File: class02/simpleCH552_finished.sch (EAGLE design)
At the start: 15 parts, among them U1 CH552G, X1 USBPCB

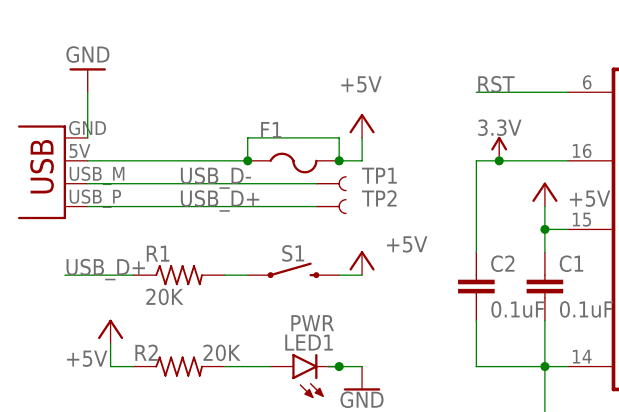
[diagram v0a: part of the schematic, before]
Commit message: remove fuse and test point
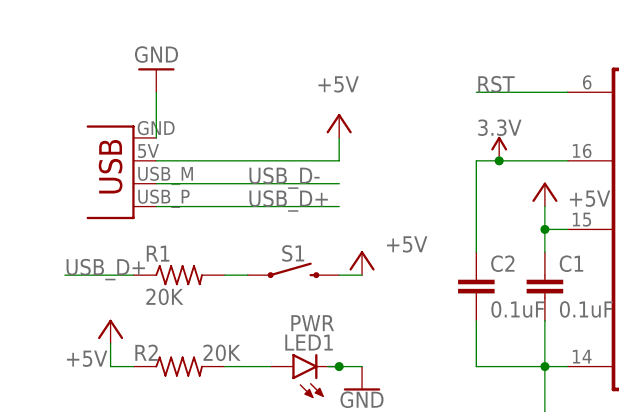
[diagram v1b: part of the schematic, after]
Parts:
- removed F1: DNP, adafruit:PTCFUSE-1206
- removed TP1, TP2: TEST-POINT3X4, SparkFun-Connectors:TEST-POINT3X4
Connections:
- net +5V: no longer F1.1, F1.2
- net USB_D+: no longer TP2.1
- net USB_D-: no longer TP1.1
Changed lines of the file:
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@@
 <attribute name="LCSC" value="C16834"/>
-</part>
-<part name="F1" library="adafruit" library_urn="urn:adsk.eagle:library:420" deviceset="PTCFUSE" device="-1206" value="DNP">
-<attribute name="LCSC" value="C151162"/>
 </part>
 <part name="GND1" library="SparkFun-PowerSymbols" library_urn="urn:adsk.eagle:library:530" deviceset="GND" device=""/>
@@
 <part name="P+4" library="supply1" library_urn="urn:adsk.eagle:library:371" deviceset="+5V" device=""/>
 <part name="P+5" library="supply1" library_urn="urn:adsk.eagle:library:371" deviceset="+5V" device=""/>
-<part name="TP1" library="SparkFun-Connectors" library_urn="urn:adsk.eagle:library:513" deviceset="TEST-POINT" device="3X4" package3d_urn="urn:adsk.eagle:package:38287/1"/>
-<part name="TP2" library="SparkFun-Connectors" library_urn="urn:adsk.eagle:library:513" deviceset="TEST-POINT" device="3X4" package3d_urn="urn:adsk.eagle:package:38287/1"/>
 <part name="S1" library="SparkFun-Switches" library_urn="urn:adsk.eagle:library:535" deviceset="MOMENTARY-SWITCH-SPST" device="-SMD-6.2MM-TALL" package3d_urn="urn:adsk.eagle:package:40172/1">
 <attribute name="LCSC" value="C557616"/>
@@
 <attribute name="VALUE" x="95.504" y="15.621" size="1.778" layer="96"/>
 </instance>
-<instance part="F1" gate="G$1" x="66.04" y="30.48" smashed="yes">
-<attribute name="LCSC" x="66.04" y="30.48" size="1.778" layer="96" display="off"/>
-<attribute name="NAME" x="62.23" y="35.56" size="1.778" layer="95"/>
-</instance>
 <instance part="GND1" gate="1" x="93.98" y="2.54" smashed="yes">
 <attribute name="VALUE" x="93.98" y="2.286" size="1.778" layer="96" align="top-center"/>
 </instance>
-<instance part="P+1" gate="1" x="73.66" y="38.1" smashed="yes">
-<attribute name="VALUE" x="71.12" y="40.64" size="1.778" layer="96"/>
+<instance part="P+1" gate="1" x="71.12" y="38.1" smashed="yes">
+<attribute name="VALUE" x="68.58" y="40.64" size="1.778" layer="96"/>
 </instance>
 <instance part="P+2" gate="1" x="93.98" y="30.48" smashed="yes">
@@
 <attribute name="LCSC" x="66.04" y="10.16" size="1.778" layer="96" rot="R90" display="off"/>
 </instance>
-<instance part="X1" gate="G$1" x="40.64" y="35.56" smashed="yes" rot="R180"/>
-<instance part="GND2" gate="1" x="43.18" y="43.18" smashed="yes" rot="R180">
-<attribute name="VALUE" x="45.72" y="45.72" size="1.778" layer="96" rot="R180"/>
+<instance part="X1" gate="G$1" x="48.26" y="35.56" smashed="yes" rot="R180"/>
+<instance part="GND2" gate="1" x="50.8" y="43.18" smashed="yes" rot="R180">
+<attribute name="VALUE" x="53.34" y="45.72" size="1.778" layer="96" rot="R180"/>
 </instance>
 <instance part="J1" gate="G$1" x="91.44" y="-20.32" smashed="yes">
@@
 <instance part="P+5" gate="1" x="73.66" y="22.86" smashed="yes">
 <attribute name="VALUE" x="76.2" y="22.86" size="1.778" layer="96"/>
-</instance>
-<instance part="TP1" gate="G$1" x="68.58" y="30.48" smashed="yes">
-<attribute name="NAME" x="73.66" y="30.48" size="1.778" layer="95" font="vector"/>
-</instance>
-<instance part="TP2" gate="G$1" x="68.58" y="27.94" smashed="yes">
-<attribute name="NAME" x="73.66" y="27.94" size="1.778" layer="95" font="vector"/>
 </instance>
 <instance part="S1" gate="G$1" x="66.04" y="20.32" smashed="yes">
@@
 <pinref part="X1" gate="G$1" pin="GND"/>
 <pinref part="GND2" gate="1" pin="GND"/>
-<wire x1="43.18" y1="35.56" x2="43.18" y2="40.64" width="0.1524" layer="91"/>
+<wire x1="50.8" y1="35.56" x2="50.8" y2="40.64" width="0.1524" layer="91"/>
 </segment>
 <segment>
@@
 <net name="USB_D-" class="0">
 <segment>
-<label x="53.34" y="30.48" size="1.778" layer="95"/>
+<label x="60.96" y="30.48" size="1.778" layer="95"/>
 <pinref part="X1" gate="G$1" pin="D-"/>
-<wire x1="68.58" y1="30.48" x2="43.18" y2="30.48" width="0.1524" layer="91"/>
-<pinref part="TP1" gate="G$1" pin="1"/>
+<wire x1="71.12" y1="30.48" x2="50.8" y2="30.48" width="0.1524" layer="91"/>
 </segment>
 <segment>
@@
 <net name="USB_D+" class="0">
 <segment>
-<label x="53.34" y="27.94" size="1.778" layer="95"/>
+<label x="60.96" y="27.94" size="1.778" layer="95"/>
 <pinref part="X1" gate="G$1" pin="D+"/>
-<wire x1="43.18" y1="27.94" x2="68.58" y2="27.94" width="0.1524" layer="91"/>
-<pinref part="TP2" gate="G$1" pin="1"/>
+<wire x1="50.8" y1="27.94" x2="71.12" y2="27.94" width="0.1524" layer="91"/>
 </segment>
 <segment>
@@
 <net name="+5V" class="0">
 <segment>
-<pinref part="F1" gate="G$1" pin="2"/>
-<wire x1="71.12" y1="33.02" x2="73.66" y2="33.02" width="0.1524" layer="91"/>
 <pinref part="P+1" gate="1" pin="+5V"/>
-<wire x1="73.66" y1="33.02" x2="73.66" y2="35.56" width="0.1524" layer="91"/>
 <wire x1="71.12" y1="33.02" x2="71.12" y2="35.56" width="0.1524" layer="91"/>
-<junction x="71.12" y="33.02"/>
-<wire x1="71.12" y1="35.56" x2="60.96" y2="35.56" width="0.1524" layer="91"/>
-<pinref part="F1" gate="G$1" pin="1"/>
 <pinref part="X1" gate="G$1" pin="VBUS"/>
-<wire x1="43.18" y1="33.02" x2="60.96" y2="33.02" width="0.1524" layer="91"/>
-<wire x1="60.96" y1="35.56" x2="60.96" y2="33.02" width="0.1524" layer="91"/>
-<junction x="60.96" y="33.02"/>
-</segment>
-<segment>
+<wire x1="50.8" y1="33.02" x2="71.12" y2="33.02" width="0.1524" layer="91"/>
+</segment>
+<segment>
